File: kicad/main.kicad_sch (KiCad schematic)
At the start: 16 parts, among them J1 Conn_battery, J2 AudioJack3, SW1 SW_Push, U1 TPS73101DBV, U2 ESP32-WROOM-32

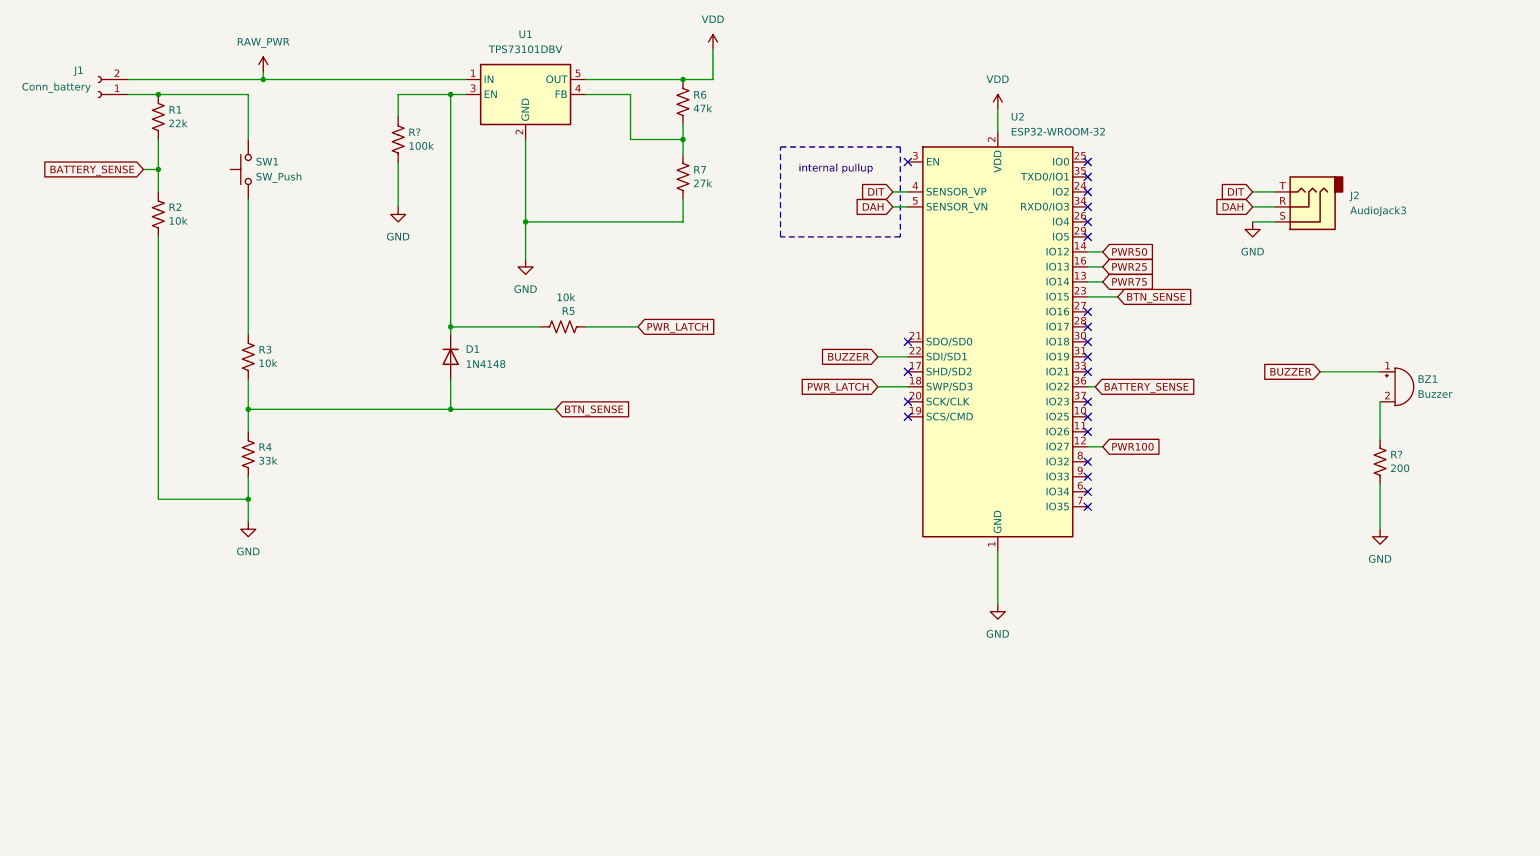
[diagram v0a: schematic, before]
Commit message: feat: schematic, pcb layout, code, enclosure
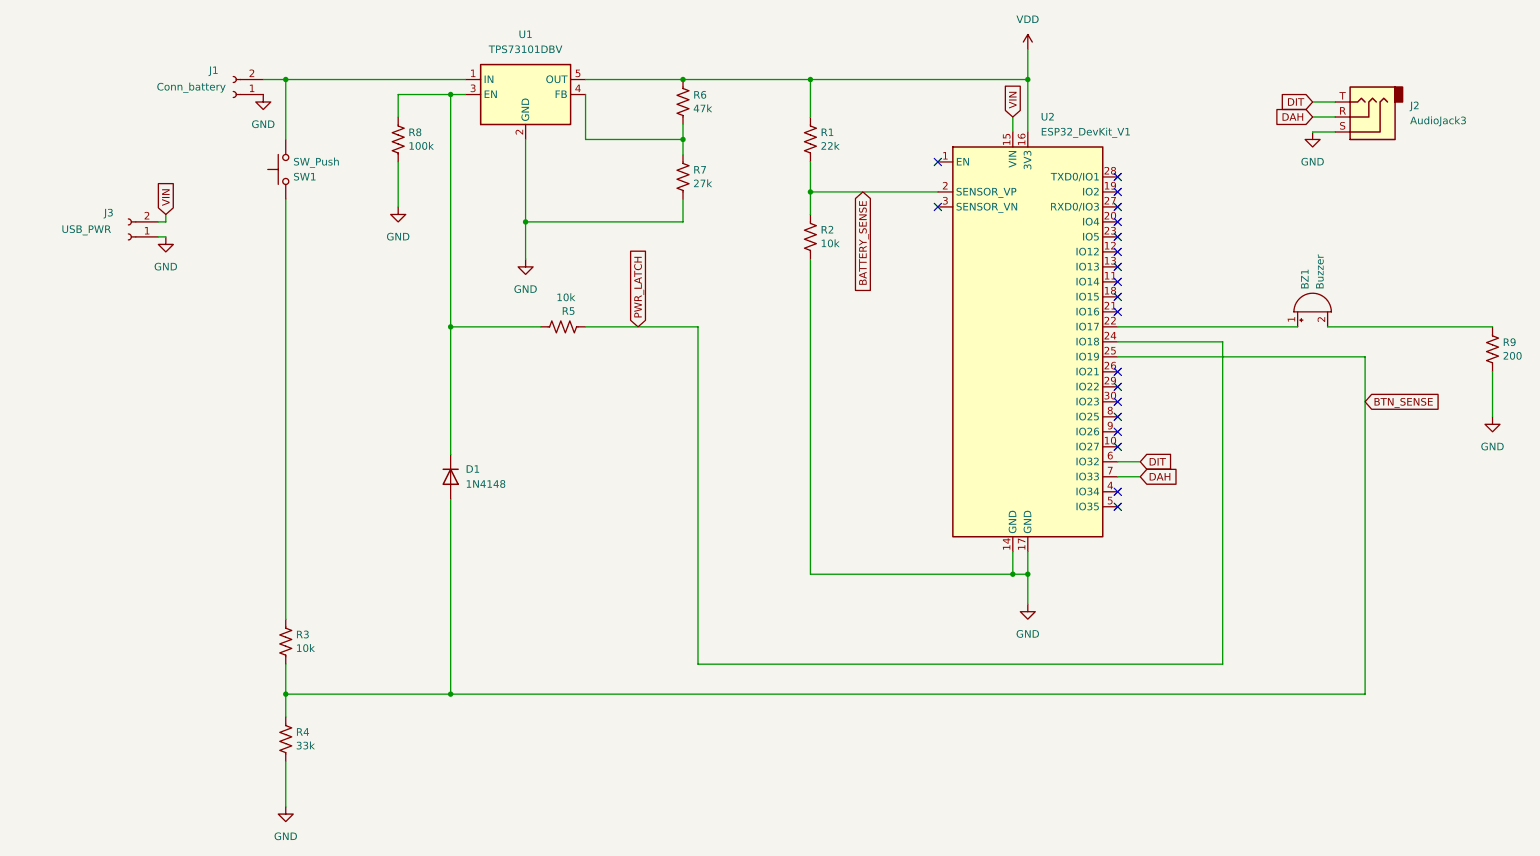
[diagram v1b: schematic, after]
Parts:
- removed U2: ESP32-WROOM-32, RF_Module:ESP32-C3-WROOM-02U, symbol RF_Module:ESP32-WROOM-32
- added J3: USB_PWR, Connector_Wire:SolderWire-1.5sqmm_1x02_P6mm_D1.7mm_OD3mm, symbol Connector:Conn_01x02_Socket
- added U2: ESP32_DevKit_V1, !my-kicad-library:esp32_devkit_v1_doit, symbol !my-kicad-library:ESP32_DevKit_V1
- BZ1: footprint (none) -> !my-kicad-library:Buzzer-GT-0905A
- D1: footprint Diode_THT:D_DO-35_SOD27_P7.62mm_Horizontal -> Diode_SMD:D_MELF
- J1: footprint (none) -> Connector_Wire:SolderWire-1.5sqmm_1x02_P6mm_D1.7mm_OD3mm
- J2: footprint (none) -> Connector_Audio:Jack_3.5mm_CUI_SJ1-3535NG_Horizontal
- SW1: footprint (none) -> Button_Switch_THT:SW_PUSH_6mm
- gave numbers to parts that had none: 2
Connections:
- net RAW_PWR is gone; now on an unnamed net: J1.2 (Pin_2), U1.1 (IN)
- net BATTERY_SENSE: now also U2.2 (SENSOR_VP)
- net BTN_SENSE: now also U2.25 (IO19)
- net DAH: now also U2.7 (IO33)
- net DIT: now also U2.6 (IO32)
- net GND: now also J1.1 (Pin_1), J3.1 (Pin_1), U2.14 (GND), U2.17 (GND)
- net PWR_LATCH: now also U2.24 (IO18)
- net VDD: now also R1.1, U2.16 (3V3)
- net at SW1.1: no longer R3.1
- net BUZZER: no longer names the net of BZ1.1 (+)
- net BUZZER: now also U2.22 (IO17)
- new net: R3.1, SW1.2
- new net VIN: J3.2 (Pin_2), U2.15 (VIN)
- no-connect marks 23 -> 20
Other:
- note removed: "internal pullup"
- moved on the sheet: BZ1, D1, J1, J2, R1, R2, R3, R4, R9, SW1
